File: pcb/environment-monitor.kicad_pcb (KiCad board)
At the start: 2 copper layers, 31.1 x 52.1 mm, 16 parts, among them P1 BME280, P2 HEADER, P3 SERIAL, P4 PWR, SW1 RESET, SW2 FLASH, U1 ESP-12E, U2 MCP1700T-3302E/TT

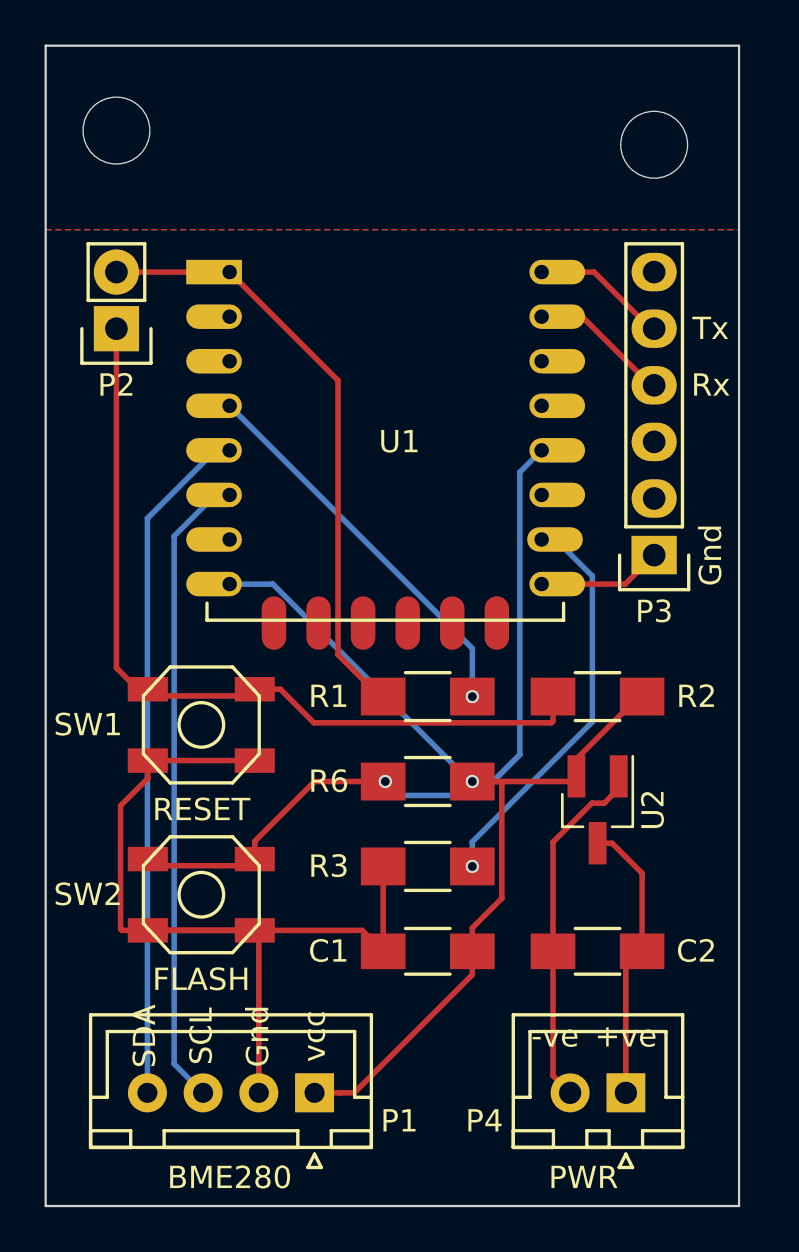
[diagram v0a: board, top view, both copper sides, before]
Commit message: Update Schematic and PCB to new design
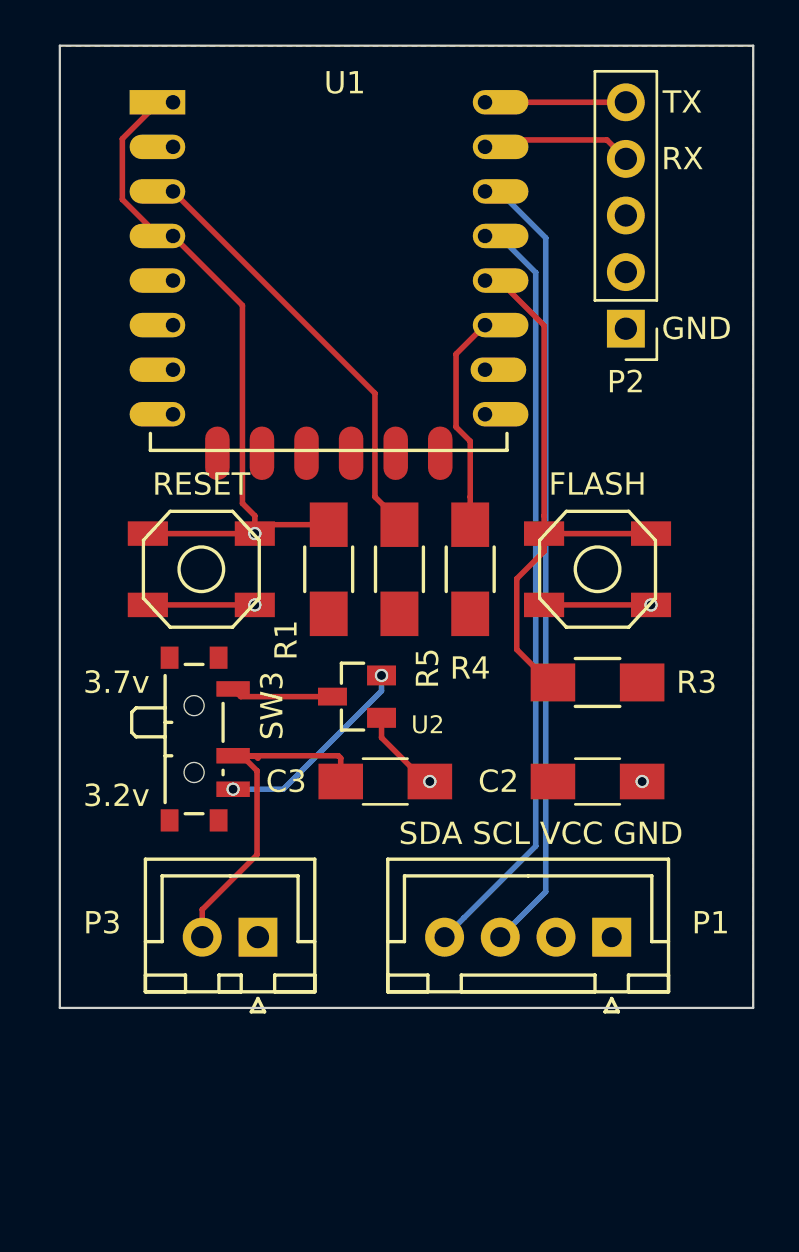
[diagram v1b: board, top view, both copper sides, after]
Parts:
- removed ? (x2): MountingHole_3mm, Mounting_Holes:MountingHole_3mm
- removed C1: 1uF, Capacitors_SMD:C_1206_HandSoldering
- removed P4: PWR, Connectors_JST:JST_XH_B02B-XH-A_02x2.50mm_Straight
- removed R2, R6: 10k, Resistors_SMD:R_1206_HandSoldering
- added C3: 1uF, Capacitors_SMD:C_1206_HandSoldering, F.Cu at (132.7, 106.7)
- added R4: 4.7k, Resistors_SMD:R_1206_HandSoldering, F.Cu at (136.5, 97.2)
- added R5: 4.7k, Resistors_SMD:R_1206_HandSoldering, F.Cu at (133.3, 97.2)
- added SW3: Switch_SPDT_x2, switches:SW_SPDT_PCM12, F.Cu at (124.5, 104.8)
- P2: value HEADER -> SERIAL; footprint Pin_Headers:Pin_Header_Straight_1x02 -> Pin_Headers:Pin_Header_Straight_1x05_Pitch2.54mm
- P3: value SERIAL -> PWR; footprint Pin_Headers:Pin_Header_Straight_1x06 -> Connectors_JST:JST_XH_B02B-XH-A_02x2.50mm_Straight
- R1: value 10R -> 4.7k
- R3: value 10k -> 4.7k
- U1: value ESP-12E -> ESP-12F
- U2: value MCP1700T-3302E/TT -> MCP1700T; footprint TO_SOT_Packages_SMD:SOT-23_Handsoldering -> smd-semi:SOT-23
- moved P3 24.7 mm to (127.0, 113.7)
- moved SW2 23.0 mm to (142.2, 97.2)
- moved P2 22.9 mm to (143.5, 86.4)
- moved P1 15.1 mm to (142.9, 113.7)
- moved U2 11.9 mm to (131.4, 102.9), turned to 180 degrees
- moved R3 11.2 mm to (142.2, 102.2)
- moved U1 8.03 mm to (123.2, 76.2)
- moved C2 7.62 mm to (142.2, 106.7), turned to 0 degrees
- moved R1 7.24 mm to (130.2, 97.2), turned to 90 degrees
- moved SW1 6.98 mm to (124.5, 97.2)
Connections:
- C2 pad 1: Net-(C2-Pad1) -> VCC
- P1 pad 1: VCC -> GND
- P1 pad 2: GND -> VCC
- P2 pad 1: Net-(P2-Pad1) -> GND
- P2 pad 2: Net-(P2-Pad2) -> (no net)
- R1 pad 1: Net-(P2-Pad2) -> VCC
- R3 pad 1: Net-(R3-Pad1) -> VCC
- R3 pad 2: GND -> /FLASH
- SW1 pad 3: Net-(P2-Pad1) -> Net-(R1-Pad2)
- SW1 pad 4: Net-(P2-Pad1) -> Net-(R1-Pad2)
- U1 pad 1: Net-(P2-Pad2) -> Net-(R1-Pad2)
- U1 pad 10: Net-(U1-Pad10) -> (no net)
- U1 pad 11: Net-(U1-Pad11) -> (no net)
- U1 pad 12: Net-(U1-Pad12) -> (no net)
- U1 pad 13: Net-(U1-Pad13) -> (no net)
- U1 pad 14: Net-(U1-Pad14) -> (no net)
- U1 pad 16: Net-(R3-Pad1) -> GND
- U1 pad 19: Net-(U1-Pad19) -> /SDA
- U1 pad 2: Net-(U1-Pad2) -> (no net)
- U1 pad 20: Net-(U1-Pad20) -> /SCL
- U1 pad 3: Net-(U1-Pad3) -> /CH_EN
- U1 pad 5: /SDA -> (no net)
- U1 pad 6: /SCL -> (no net)
- U1 pad 7: Net-(U1-Pad7) -> (no net)
- U1 pad 9: Net-(U1-Pad9) -> (no net)
- U2 pad 3: Net-(C2-Pad1) -> Net-(SW3-Pad1)
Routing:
- net GND: track 62.7 -> 13.9 mm, vias 0 -> 4
- net Net-(P2-Pad1): track 38.0 -> 0.00 mm
- net VCC: track 43.9 -> 9.18 mm, vias 1 -> 2
- net Net-(P2-Pad2): track 27.1 -> 0.00 mm
- net /CH_EN: track 0.00 -> 19.2 mm
- net Net-(R3-Pad1): track 18.8 -> 0.00 mm, vias 1 -> 0
- net Net-(C3-Pad1): track 0.00 -> 16.9 mm
- net Net-(R1-Pad2): track 17.6 -> 31.8 mm
- net Net-(C2-Pad1): track 13.9 -> 0.00 mm
- net Net-(R4-Pad2): track 0.00 -> 10.3 mm
- net /FLASH: track 33.7 -> 25.6 mm, vias 1 -> 0
- net /SCL: track 28.8 -> 35.8 mm
- net Net-(SW3-Pad1): track 0.00 -> 4.60 mm
- net /SDA: track 30.7 -> 34.5 mm
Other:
- board size 31.1 x 52.1 mm -> 31.1 x 43.2 mm
- board text added: "3.2v"
- board text added: "3.7v"
- board text added: "Environment Monitor v1.4 Alan Lord 2017"
- board text added: "GND"
- board text added: "RX"
- board text added: "SDA SCL VCC GND"
- board text added: "TX"
- board text removed: "+ve"
- board text removed: "-ve"
- board text removed: "BME280"
- board text removed: "Environment Monitor v1.2 Alan Lord 2017"
- board text removed: "Gnd"
- board text removed: "PWR"
- board text removed: "Rx"
- board text removed: "SCL"
- board text removed: "SDA"
- board text removed: "Tx"
- board text removed: "vcc"
